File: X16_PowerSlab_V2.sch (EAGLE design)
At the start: 37 parts, among them J4 796636-6

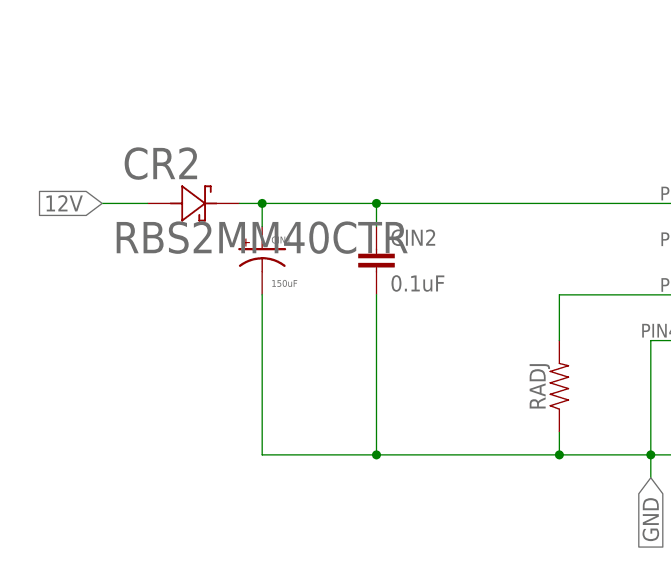
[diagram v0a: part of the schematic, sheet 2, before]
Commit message: Minh update 4
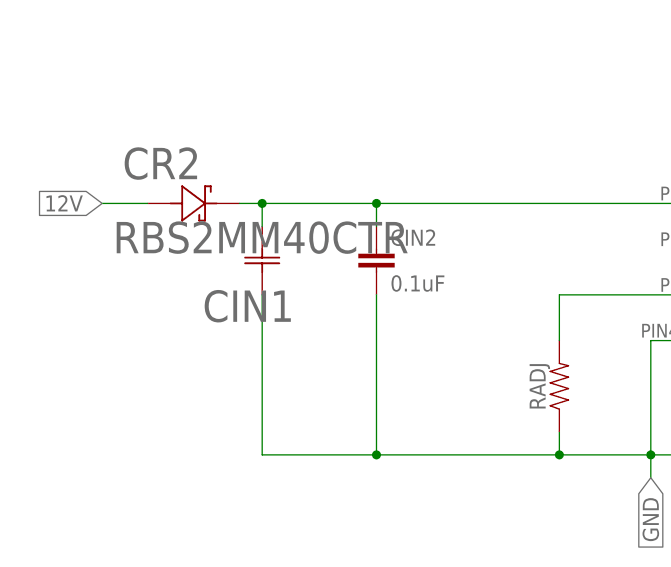
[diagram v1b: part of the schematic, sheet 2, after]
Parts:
- CIN1: value 150uF -> 594D187X0016R2T; device X15-Conversion-Parts-Library:C-TANTALUM(10UF_150UF) -> X16_Power_Slab:594D187X0016R2T
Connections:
- net GND: now also CIN1.2; no longer CIN1.-
- net VIN: now also CIN1.1; no longer CIN1.+
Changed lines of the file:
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@@
 <part name="COUT5" library="X15-Conversion-Parts-Library" deviceset="C-TANTALUM(10UF_150UF)" device="" package3d_urn="urn:adsk.eagle:package:25131320/3" value="150uF"/>
 <part name="COUT6" library="X15-Conversion-Parts-Library" deviceset="C-TANTALUM(10UF_150UF)" device="" package3d_urn="urn:adsk.eagle:package:25131320/3" value="150uF"/>
-<part name="CIN1" library="X15-Conversion-Parts-Library" deviceset="C-TANTALUM(10UF_150UF)" device="" package3d_urn="urn:adsk.eagle:package:25131320/3" value="150uF"/>
 <part name="CR2" library="X16_Power_Slab" deviceset="RBS2MM40CTR" device=""/>
 <part name="48V" library="X16-ExtraComponents" deviceset="TESTPOINT_5.04MM" device="" value="48V"/>
@@
 <part name="R3" library="SparkFun-Resistors" library_urn="urn:adsk.eagle:library:532" deviceset="0.1OHM" device="-0603-1/3W-1%" package3d_urn="urn:adsk.eagle:package:41389018/1" value="150k"/>
 <part name="R5" library="SparkFun-Resistors" library_urn="urn:adsk.eagle:library:532" deviceset="0.1OHM" device="-0603-1/3W-1%" package3d_urn="urn:adsk.eagle:package:41389018/1" value="220k"/>
+<part name="CIN1" library="X16_Power_Slab" deviceset="594D187X0016R2T" device=""/>
 </parts>
 <sheets>
@@
 <attribute name="VALUE" x="82.296" y="46.609" size="0.762" layer="96"/>
 </instance>
-<instance part="CIN1" gate="G$1" x="-60.96" y="66.04" smashed="yes">
-<attribute name="NAME" x="-59.944" y="66.675" size="0.762" layer="95"/>
-<attribute name="VALUE" x="-59.944" y="61.849" size="0.762" layer="96"/>
-</instance>
 <instance part="CR2" gate="A" x="-73.66" y="71.12" smashed="yes">
 <attribute name="VALUE" x="-77.5462" y="65.5828" size="3.4798" layer="96" ratio="10" rot="SR0"/>
 <attribute name="NAME" x="-76.4794" y="73.8124" size="3.4798" layer="95" ratio="10" rot="SR0"/>
+</instance>
+<instance part="CIN1" gate="A" x="-60.96" y="68.58" smashed="yes" rot="R270">
+<attribute name="VALUE" x="-84.2772" y="58.4962" size="3.4798" layer="96" ratio="10" rot="SR270" display="off"/>
+<attribute name="NAME" x="-67.5894" y="57.9628" size="3.4798" layer="95" ratio="10" rot="SR0"/>
 </instance>
 </instances>
@@
 <pinref part="COUT5" gate="G$1" pin="-"/>
 <pinref part="COUT6" gate="G$1" pin="-"/>
-<pinref part="CIN1" gate="G$1" pin="-"/>
+<pinref part="CIN1" gate="A" pin="2"/>
 </segment>
 </net>
@@
 <junction x="-48.26" y="71.12"/>
 <wire x1="-48.26" y1="71.12" x2="-15.24" y2="71.12" width="0.1524" layer="91"/>
-<pinref part="CIN1" gate="G$1" pin="+"/>
 <pinref part="CR2" gate="A" pin="1"/>
 <wire x1="-63.5" y1="71.12" x2="-60.96" y2="71.12" width="0.1524" layer="91"/>
 <junction x="-60.96" y="71.12"/>
-</segment>
-</net>
+<pinref part="CIN1" gate="A" pin="1"/>
+</segment>
+</net>
